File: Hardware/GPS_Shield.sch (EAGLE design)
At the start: 52 parts, among them J1 ARDUINO_R3_SHIELD, J2 USD_CONNECTOR, U1 APK2112-3.3V, U2 GP3906-TLP, U3 TXB0108

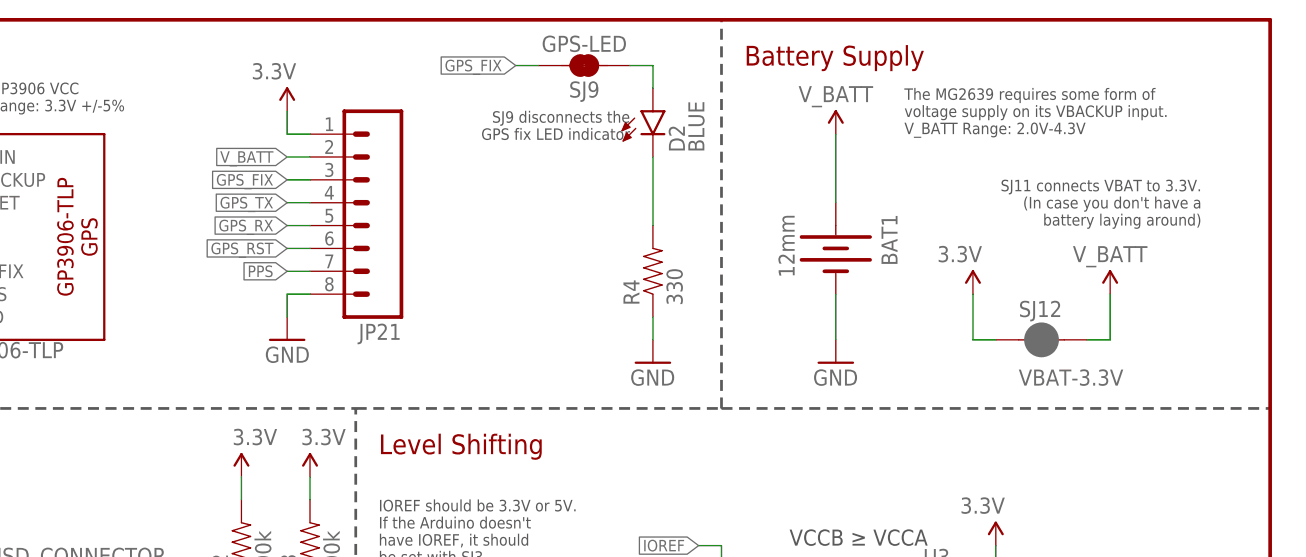
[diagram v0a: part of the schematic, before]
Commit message: Schematic cleanup
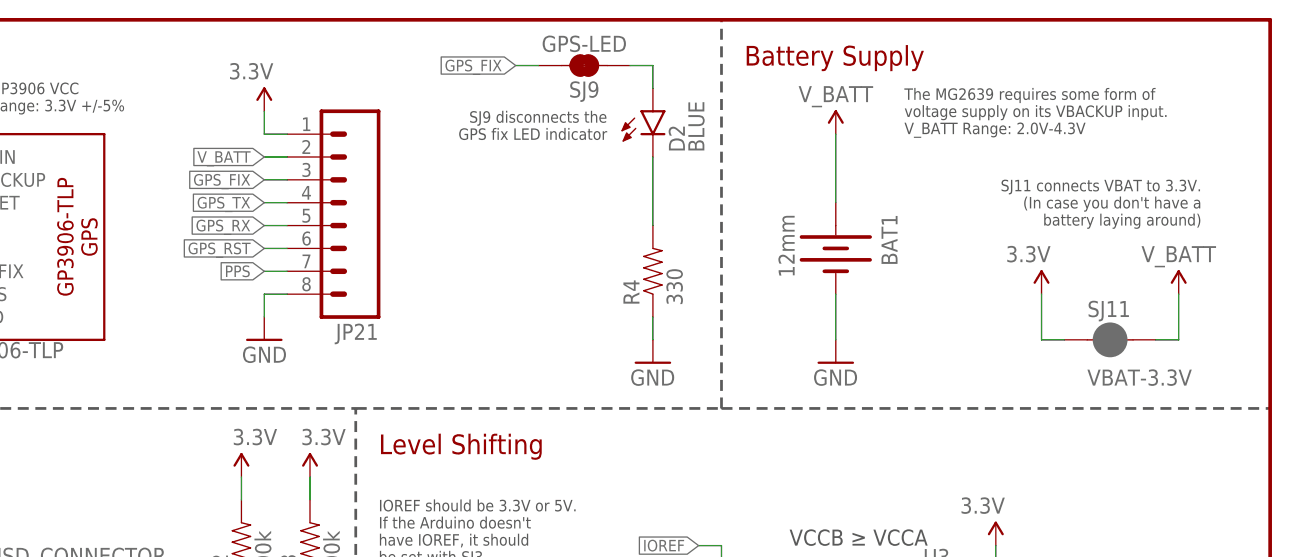
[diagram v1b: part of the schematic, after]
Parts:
- removed SJ12: VBAT-3.3V, SparkFun-Passives:JUMPER-PAD-2-NC_BY_PASTE
- added SJ11: VBAT-3.3V, SparkFun-Passives:JUMPER-PAD-2-NC_BY_PASTE
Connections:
- net 3.3V: now also SJ11.1; no longer SJ12.1
- net V_BATT: now also SJ11.2; no longer SJ12.2
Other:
- moved on the sheet: JP21
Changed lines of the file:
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@@
 <part name="P+13" library="SparkFun" deviceset="3.3V" device=""/>
 <part name="GND19" library="SparkFun" deviceset="GND" device=""/>
-<part name="SJ12" library="SparkFun-Passives" deviceset="JUMPER-PAD-2-NC_BY_PASTE" device="" value="VBAT-3.3V"/>
+<part name="SJ11" library="SparkFun-Passives" deviceset="JUMPER-PAD-2-NC_BY_PASTE" device="" value="VBAT-3.3V"/>
 </parts>
 <sheets>
@@
 the power LED
 indicator</text>
-<text x="177.8" y="175.26" size="1.27" layer="97" rot="MR0" align="top-left">SJ9 disconnects the
+<text x="175.26" y="175.26" size="1.27" layer="97" rot="MR0" align="top-left">SJ9 disconnects the
 GPS fix LED indicator</text>
 <text x="17.78" y="60.96" size="1.27" layer="97" align="top-left">SJ2 selects 3.3V
@@
 <instance part="P+6" gate="G$1" x="134.62" y="134.62"/>
 <instance part="P+7" gate="G$1" x="142.24" y="134.62"/>
-<instance part="P+12" gate="G$1" x="215.9" y="154.94" rot="MR0"/>
-<instance part="SUPPLY7" gate="G$1" x="231.14" y="154.94" smashed="yes">
-<attribute name="VALUE" x="231.14" y="158.496" size="1.778" layer="96" align="bottom-center"/>
-</instance>
-<instance part="JP21" gate="G$1" x="147.32" y="165.1" rot="R180"/>
-<instance part="P+13" gate="G$1" x="139.7" y="175.26" rot="MR0"/>
-<instance part="GND19" gate="1" x="139.7" y="149.86" rot="MR0"/>
-<instance part="SJ12" gate="G$1" x="223.52" y="149.86"/>
+<instance part="P+12" gate="G$1" x="223.52" y="154.94" rot="MR0"/>
+<instance part="SUPPLY7" gate="G$1" x="238.76" y="154.94" smashed="yes">
+<attribute name="VALUE" x="238.76" y="158.496" size="1.778" layer="96" align="bottom-center"/>
+</instance>
+<instance part="JP21" gate="G$1" x="144.78" y="165.1" rot="R180"/>
+<instance part="P+13" gate="G$1" x="137.16" y="175.26" rot="MR0"/>
+<instance part="GND19" gate="1" x="137.16" y="149.86" rot="MR0"/>
+<instance part="SJ11" gate="G$1" x="231.14" y="149.86"/>
 </instances>
 <busses>
@@
 <segment>
 <pinref part="JP21" gate="G$1" pin="8"/>
-<wire x1="142.24" y1="154.94" x2="139.7" y2="154.94" width="0.1524" layer="91"/>
-<wire x1="139.7" y1="154.94" x2="139.7" y2="152.4" width="0.1524" layer="91"/>
+<wire x1="139.7" y1="154.94" x2="137.16" y2="154.94" width="0.1524" layer="91"/>
+<wire x1="137.16" y1="154.94" x2="137.16" y2="152.4" width="0.1524" layer="91"/>
 <pinref part="GND19" gate="1" pin="GND"/>
 </segment>
@@
 <segment>
 <pinref part="P+12" gate="G$1" pin="3.3V"/>
-<wire x1="218.44" y1="149.86" x2="215.9" y2="149.86" width="0.1524" layer="91"/>
-<wire x1="215.9" y1="149.86" x2="215.9" y2="154.94" width="0.1524" layer="91"/>
-<pinref part="SJ12" gate="G$1" pin="1"/>
+<wire x1="226.06" y1="149.86" x2="223.52" y2="149.86" width="0.1524" layer="91"/>
+<wire x1="223.52" y1="149.86" x2="223.52" y2="154.94" width="0.1524" layer="91"/>
+<pinref part="SJ11" gate="G$1" pin="1"/>
 </segment>
 <segment>
 <pinref part="JP21" gate="G$1" pin="1"/>
-<wire x1="142.24" y1="172.72" x2="139.7" y2="172.72" width="0.1524" layer="91"/>
-<wire x1="139.7" y1="172.72" x2="139.7" y2="175.26" width="0.1524" layer="91"/>
+<wire x1="139.7" y1="172.72" x2="137.16" y2="172.72" width="0.1524" layer="91"/>
+<wire x1="137.16" y1="172.72" x2="137.16" y2="175.26" width="0.1524" layer="91"/>
 <pinref part="P+13" gate="G$1" pin="3.3V"/>
 </segment>
@@
 <segment>
 <pinref part="JP21" gate="G$1" pin="7"/>
-<wire x1="142.24" y1="157.48" x2="139.7" y2="157.48" width="0.1524" layer="91"/>
-<label x="139.7" y="157.48" size="1.27" layer="95" rot="R180" xref="yes"/>
+<wire x1="139.7" y1="157.48" x2="137.16" y2="157.48" width="0.1524" layer="91"/>
+<label x="137.16" y="157.48" size="1.27" layer="95" rot="R180" xref="yes"/>
 </segment>
 </net>
@@
 <segment>
 <pinref part="SUPPLY7" gate="G$1" pin="V_BATT"/>
-<wire x1="228.6" y1="149.86" x2="231.14" y2="149.86" width="0.1524" layer="91"/>
-<wire x1="231.14" y1="149.86" x2="231.14" y2="154.94" width="0.1524" layer="91"/>
-<pinref part="SJ12" gate="G$1" pin="2"/>
+<wire x1="236.22" y1="149.86" x2="238.76" y2="149.86" width="0.1524" layer="91"/>
+<wire x1="238.76" y1="149.86" x2="238.76" y2="154.94" width="0.1524" layer="91"/>
+<pinref part="SJ11" gate="G$1" pin="2"/>
 </segment>
 <segment>
@@
 <segment>
 <pinref part="JP21" gate="G$1" pin="2"/>
-<wire x1="142.24" y1="170.18" x2="139.7" y2="170.18" width="0.1524" layer="91"/>
-<label x="139.7" y="170.18" size="1.27" layer="95" rot="R180" xref="yes"/>
+<wire x1="139.7" y1="170.18" x2="137.16" y2="170.18" width="0.1524" layer="91"/>
+<label x="137.16" y="170.18" size="1.27" layer="95" rot="R180" xref="yes"/>
 </segment>
 </net>
@@
 <segment>
 <pinref part="JP21" gate="G$1" pin="5"/>
-<wire x1="142.24" y1="162.56" x2="139.7" y2="162.56" width="0.1524" layer="91"/>
-<label x="139.7" y="162.56" size="1.27" layer="95" rot="R180" xref="yes"/>
+<wire x1="139.7" y1="162.56" x2="137.16" y2="162.56" width="0.1524" layer="91"/>
+<label x="137.16" y="162.56" size="1.27" layer="95" rot="R180" xref="yes"/>
 </segment>
 </net>
@@
 <segment>
 <pinref part="JP21" gate="G$1" pin="4"/>
-<wire x1="142.24" y1="165.1" x2="139.7" y2="165.1" width="0.1524" layer="91"/>
-<label x="139.7" y="165.1" size="1.27" layer="95" rot="R180" xref="yes"/>
+<wire x1="139.7" y1="165.1" x2="137.16" y2="165.1" width="0.1524" layer="91"/>
+<label x="137.16" y="165.1" size="1.27" layer="95" rot="R180" xref="yes"/>
 </segment>
 </net>
@@
 <segment>
 <pinref part="JP21" gate="G$1" pin="3"/>
-<wire x1="142.24" y1="167.64" x2="139.7" y2="167.64" width="0.1524" layer="91"/>
-<label x="139.7" y="167.64" size="1.27" layer="95" rot="R180" xref="yes"/>
+<wire x1="139.7" y1="167.64" x2="137.16" y2="167.64" width="0.1524" layer="91"/>
+<label x="137.16" y="167.64" size="1.27" layer="95" rot="R180" xref="yes"/>
 </segment>
 </net>
@@
 <segment>
 <pinref part="JP21" gate="G$1" pin="6"/>
-<wire x1="142.24" y1="160.02" x2="139.7" y2="160.02" width="0.1524" layer="91"/>
-<label x="139.7" y="160.02" size="1.27" layer="95" rot="R180" xref="yes"/>
-</segment>
-</net>
+<wire x1="139.7" y1="160.02" x2="137.16" y2="160.02" width="0.1524" layer="91"/>
+<label x="137.16" y="160.02" size="1.27" layer="95" rot="R180" xref="yes"/>
+</segment>
+</net>
